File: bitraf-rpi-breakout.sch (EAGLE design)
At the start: 20 parts, among them IC1 74HC595N, K1 FTR-F3FTR-F3AA005E, T1 BC547

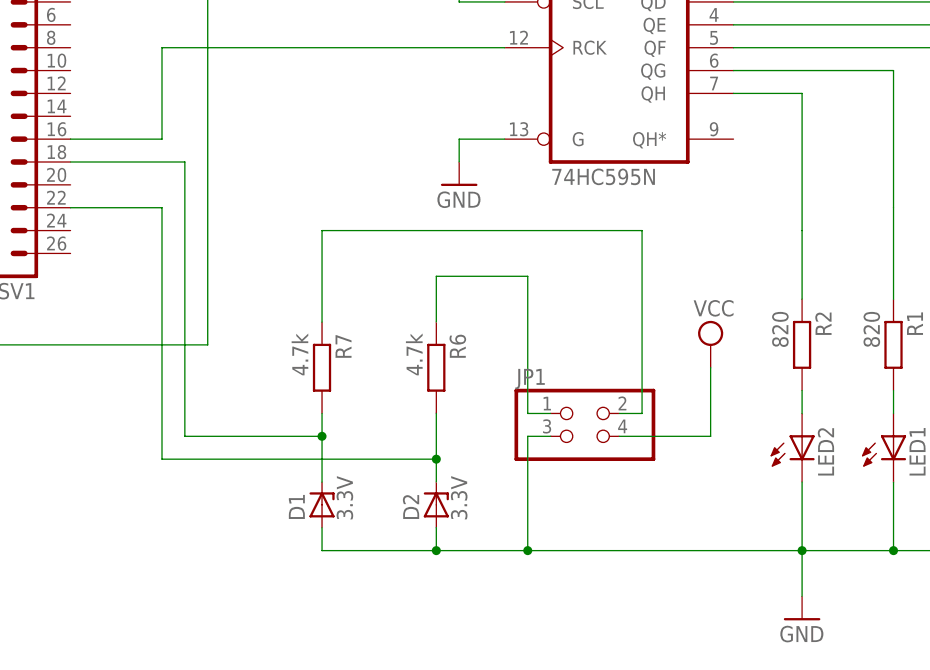
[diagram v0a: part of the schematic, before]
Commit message: o Rev D.
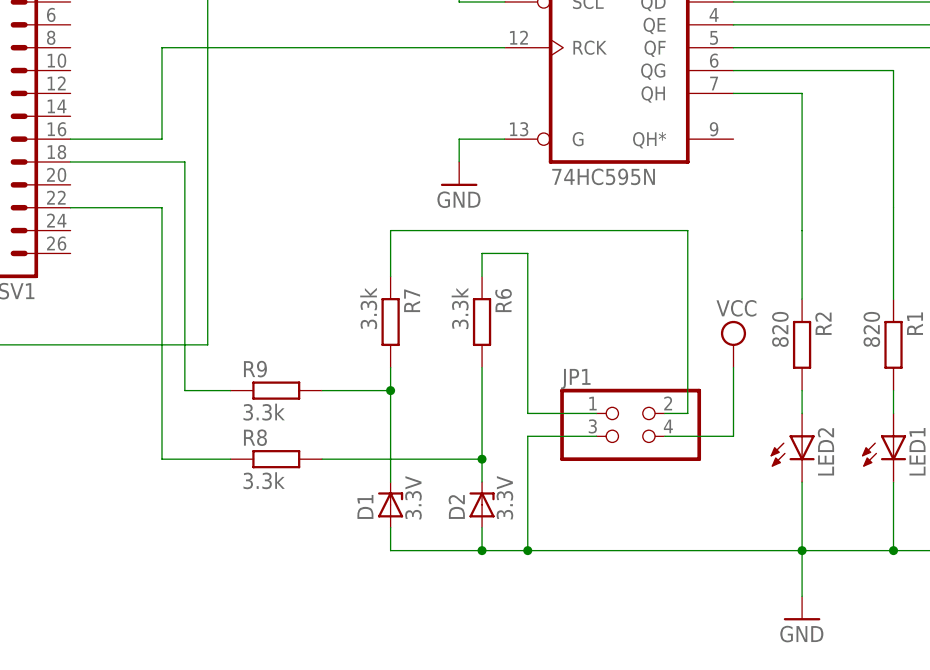
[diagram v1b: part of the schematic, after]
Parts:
- added R8, R9: 3.3k, resistor:R-EU_0204/7
- R6, R7: value 4.7k -> 3.3k
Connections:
- new net N$11: D1.C, R7.2, R9.2
- new net N$18: D2.C, R6.2, R8.2
- net N$8: now also R8.1; no longer D2.C, R6.2
- net N$9: now also R9.1; no longer D1.C, R7.2
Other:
- moved on the sheet: D1, D2, JP1, R6, R7
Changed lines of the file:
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@@
 <part name="R5" library="resistor" deviceset="R-EU_" device="0204/7" value="1k"/>
 <part name="GND2" library="supply1" deviceset="GND" device=""/>
-<part name="R6" library="resistor" deviceset="R-EU_" device="0204/7" value="4.7k"/>
-<part name="R7" library="resistor" deviceset="R-EU_" device="0204/7" value="4.7k"/>
+<part name="R6" library="resistor" deviceset="R-EU_" device="0204/7" value="3.3k"/>
+<part name="R7" library="resistor" deviceset="R-EU_" device="0204/7" value="3.3k"/>
 <part name="SUPPLY1" library="supply2" deviceset="VCC" device=""/>
 <part name="D3" library="diode" deviceset="1N4004" device=""/>
@@
 <part name="SUPPLY4" library="supply2" deviceset="VCC" device=""/>
 <part name="K1" library="fujitsu-ftr-f3" deviceset="FTR-F3" device="" technology="FTR-F3AA005E"/>
+<part name="R8" library="resistor" deviceset="R-EU_" device="0204/7" value="3.3k"/>
+<part name="R9" library="resistor" deviceset="R-EU_" device="0204/7" value="3.3k"/>
 </parts>
 <sheets>
@@
 <instance part="R3" gate="G$1" x="119.38" y="48.26" rot="R270"/>
 <instance part="R4" gate="G$1" x="109.22" y="48.26" rot="R270"/>
-<instance part="D1" gate="G$1" x="35.56" y="30.48" rot="R90"/>
-<instance part="D2" gate="G$1" x="48.26" y="30.48" rot="R90"/>
+<instance part="D1" gate="G$1" x="43.18" y="30.48" rot="R90"/>
+<instance part="D2" gate="G$1" x="53.34" y="30.48" rot="R90"/>
 <instance part="LED1" gate="G$1" x="99.06" y="38.1"/>
 <instance part="LED2" gate="G$1" x="88.9" y="38.1"/>
@@
 <instance part="R5" gate="G$1" x="147.32" y="35.56"/>
 <instance part="GND2" gate="1" x="160.02" y="17.78"/>
-<instance part="R6" gate="G$1" x="48.26" y="45.72" rot="R270"/>
-<instance part="R7" gate="G$1" x="35.56" y="45.72" rot="R270"/>
+<instance part="R6" gate="G$1" x="53.34" y="50.8" rot="R270"/>
+<instance part="R7" gate="G$1" x="43.18" y="50.8" rot="R270"/>
 <instance part="SUPPLY1" gate="G$1" x="160.02" y="101.6"/>
 <instance part="D3" gate="1" x="147.32" y="60.96" rot="R90"/>
@@
 <instance part="GND3" gate="1" x="-10.16" y="53.34"/>
 <instance part="GND4" gate="1" x="50.8" y="66.04"/>
-<instance part="JP1" gate="A" x="66.04" y="38.1"/>
+<instance part="JP1" gate="A" x="71.12" y="38.1"/>
 <instance part="J1" gate="G$1" x="208.28" y="60.96" rot="MR90"/>
-<instance part="SUPPLY3" gate="G$1" x="78.74" y="48.26"/>
+<instance part="SUPPLY3" gate="G$1" x="81.28" y="48.26"/>
 <instance part="SUPPLY4" gate="G$1" x="50.8" y="99.06"/>
 <instance part="K1" gate="1" x="160.02" y="60.96"/>
 <instance part="K1" gate="2" x="177.8" y="60.96"/>
+<instance part="R8" gate="G$1" x="30.48" y="35.56"/>
+<instance part="R9" gate="G$1" x="30.48" y="43.18"/>
 </instances>
 <busses>
@@
 <pinref part="D1" gate="G$1" pin="A"/>
 <wire x1="88.9" y1="25.4" x2="58.42" y2="25.4" width="0.1524" layer="91"/>
-<wire x1="58.42" y1="25.4" x2="48.26" y2="25.4" width="0.1524" layer="91"/>
-<wire x1="48.26" y1="25.4" x2="35.56" y2="25.4" width="0.1524" layer="91"/>
-<wire x1="35.56" y1="25.4" x2="35.56" y2="27.94" width="0.1524" layer="91"/>
+<wire x1="58.42" y1="25.4" x2="53.34" y2="25.4" width="0.1524" layer="91"/>
+<wire x1="53.34" y1="25.4" x2="43.18" y2="25.4" width="0.1524" layer="91"/>
+<wire x1="43.18" y1="25.4" x2="43.18" y2="27.94" width="0.1524" layer="91"/>
 <pinref part="D2" gate="G$1" pin="A"/>
-<wire x1="48.26" y1="25.4" x2="48.26" y2="27.94" width="0.1524" layer="91"/>
-<junction x="48.26" y="25.4"/>
+<wire x1="53.34" y1="25.4" x2="53.34" y2="27.94" width="0.1524" layer="91"/>
+<junction x="53.34" y="25.4"/>
 <pinref part="LED4" gate="G$1" pin="C"/>
 <wire x1="99.06" y1="25.4" x2="109.22" y2="25.4" width="0.1524" layer="91"/>
@@
 <junction x="109.22" y="25.4"/>
 <pinref part="JP1" gate="A" pin="3"/>
-<wire x1="60.96" y1="38.1" x2="58.42" y2="38.1" width="0.1524" layer="91"/>
+<wire x1="66.04" y1="38.1" x2="58.42" y2="38.1" width="0.1524" layer="91"/>
 <wire x1="58.42" y1="38.1" x2="58.42" y2="25.4" width="0.1524" layer="91"/>
 <junction x="58.42" y="25.4"/>
@@
 <net name="N$9" class="0">
 <segment>
-<wire x1="20.32" y1="38.1" x2="20.32" y2="68.58" width="0.1524" layer="91"/>
 <pinref part="SV1" gate="1" pin="18"/>
+<wire x1="20.32" y1="43.18" x2="20.32" y2="68.58" width="0.1524" layer="91"/>
 <wire x1="20.32" y1="68.58" x2="7.62" y2="68.58" width="0.1524" layer="91"/>
-<wire x1="20.32" y1="38.1" x2="35.56" y2="38.1" width="0.1524" layer="91"/>
-<pinref part="D1" gate="G$1" pin="C"/>
-<pinref part="R7" gate="G$1" pin="2"/>
-<wire x1="35.56" y1="40.64" x2="35.56" y2="38.1" width="0.1524" layer="91"/>
-<junction x="35.56" y="38.1"/>
-<wire x1="35.56" y1="38.1" x2="35.56" y2="33.02" width="0.1524" layer="91"/>
+<pinref part="R9" gate="G$1" pin="1"/>
+<wire x1="20.32" y1="43.18" x2="25.4" y2="43.18" width="0.1524" layer="91"/>
 </segment>
 </net>
@@
 <segment>
 <pinref part="R6" gate="G$1" pin="1"/>
-<wire x1="48.26" y1="50.8" x2="48.26" y2="55.88" width="0.1524" layer="91"/>
-<wire x1="48.26" y1="55.88" x2="58.42" y2="55.88" width="0.1524" layer="91"/>
+<wire x1="53.34" y1="55.88" x2="53.34" y2="58.42" width="0.1524" layer="91"/>
+<wire x1="53.34" y1="58.42" x2="58.42" y2="58.42" width="0.1524" layer="91"/>
 <pinref part="JP1" gate="A" pin="1"/>
-<wire x1="60.96" y1="40.64" x2="58.42" y2="40.64" width="0.1524" layer="91"/>
-<wire x1="58.42" y1="40.64" x2="58.42" y2="55.88" width="0.1524" layer="91"/>
+<wire x1="66.04" y1="40.64" x2="58.42" y2="40.64" width="0.1524" layer="91"/>
+<wire x1="58.42" y1="40.64" x2="58.42" y2="58.42" width="0.1524" layer="91"/>
 </segment>
 </net>
@@
 <segment>
 <pinref part="R7" gate="G$1" pin="1"/>
-<wire x1="35.56" y1="50.8" x2="35.56" y2="60.96" width="0.1524" layer="91"/>
+<wire x1="43.18" y1="55.88" x2="43.18" y2="60.96" width="0.1524" layer="91"/>
 <pinref part="JP1" gate="A" pin="2"/>
-<wire x1="68.58" y1="40.64" x2="71.12" y2="40.64" width="0.1524" layer="91"/>
-<wire x1="71.12" y1="40.64" x2="71.12" y2="60.96" width="0.1524" layer="91"/>
-<wire x1="71.12" y1="60.96" x2="35.56" y2="60.96" width="0.1524" layer="91"/>
+<wire x1="73.66" y1="40.64" x2="76.2" y2="40.64" width="0.1524" layer="91"/>
+<wire x1="76.2" y1="40.64" x2="76.2" y2="60.96" width="0.1524" layer="91"/>
+<wire x1="76.2" y1="60.96" x2="43.18" y2="60.96" width="0.1524" layer="91"/>
 </segment>
 </net>
@@
 <segment>
 <pinref part="JP1" gate="A" pin="4"/>
-<wire x1="68.58" y1="38.1" x2="78.74" y2="38.1" width="0.1524" layer="91"/>
-<wire x1="78.74" y1="38.1" x2="78.74" y2="45.72" width="0.1524" layer="91"/>
+<wire x1="73.66" y1="38.1" x2="81.28" y2="38.1" width="0.1524" layer="91"/>
+<wire x1="81.28" y1="38.1" x2="81.28" y2="45.72" width="0.1524" layer="91"/>
 <pinref part="SUPPLY3" gate="G$1" pin="VCC"/>
 </segment>
@@
 <wire x1="7.62" y1="63.5" x2="17.78" y2="63.5" width="0.1524" layer="91"/>
 <wire x1="17.78" y1="63.5" x2="17.78" y2="35.56" width="0.1524" layer="91"/>
+<pinref part="R8" gate="G$1" pin="1"/>
+<wire x1="17.78" y1="35.56" x2="25.4" y2="35.56" width="0.1524" layer="91"/>
+</segment>
+</net>
+<net name="N$11" class="0">
+<segment>
+<pinref part="D1" gate="G$1" pin="C"/>
+<pinref part="R7" gate="G$1" pin="2"/>
+<wire x1="43.18" y1="45.72" x2="43.18" y2="43.18" width="0.1524" layer="91"/>
+<pinref part="R9" gate="G$1" pin="2"/>
+<wire x1="43.18" y1="43.18" x2="43.18" y2="33.02" width="0.1524" layer="91"/>
+<wire x1="35.56" y1="43.18" x2="43.18" y2="43.18" width="0.1524" layer="91"/>
+<junction x="43.18" y="43.18"/>
+</segment>
+</net>
+<net name="N$18" class="0">
+<segment>
 <pinref part="D2" gate="G$1" pin="C"/>
 <pinref part="R6" gate="G$1" pin="2"/>
-<wire x1="48.26" y1="40.64" x2="48.26" y2="35.56" width="0.1524" layer="91"/>
-<wire x1="48.26" y1="35.56" x2="48.26" y2="33.02" width="0.1524" layer="91"/>
-<wire x1="17.78" y1="35.56" x2="48.26" y2="35.56" width="0.1524" layer="91"/>
-<junction x="48.26" y="35.56"/>
-</segment>
-</net>
+<wire x1="53.34" y1="45.72" x2="53.34" y2="35.56" width="0.1524" layer="91"/>
+<pinref part="R8" gate="G$1" pin="2"/>
+<wire x1="53.34" y1="35.56" x2="53.34" y2="33.02" width="0.1524" layer="91"/>
+<wire x1="35.56" y1="35.56" x2="53.34" y2="35.56" width="0.1524" layer="91"/>
+<junction x="53.34" y="35.56"/>
+</segment>
+</net>
